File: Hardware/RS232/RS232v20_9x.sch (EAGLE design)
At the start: 13 parts, among them U1 SP3232XTSSOP

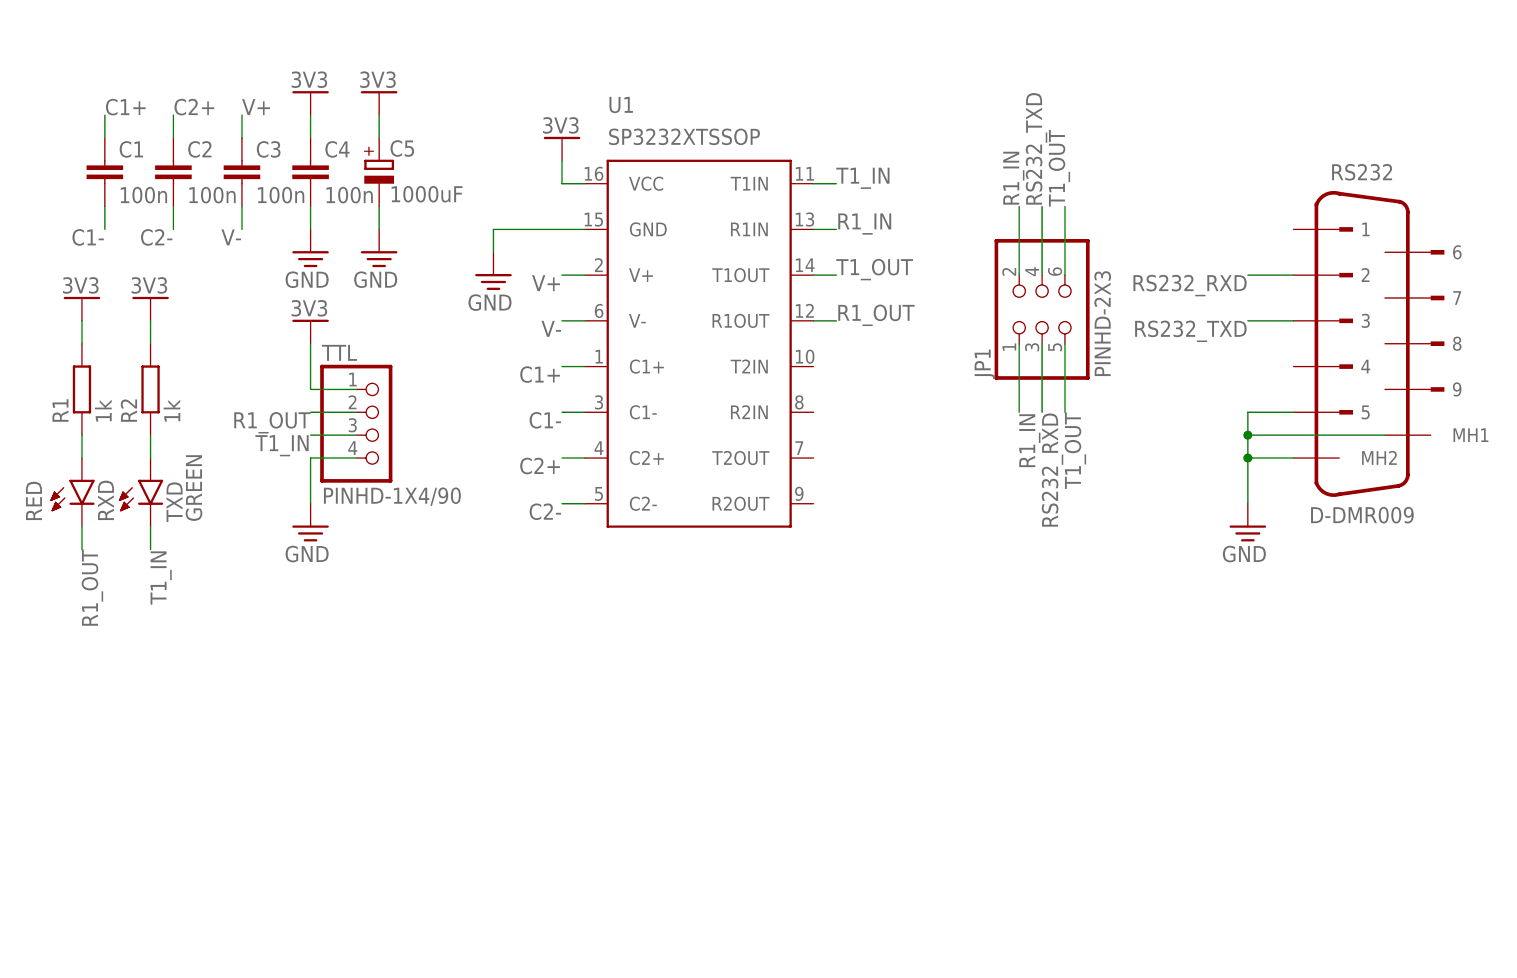
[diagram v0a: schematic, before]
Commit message: RS232 & Powder List
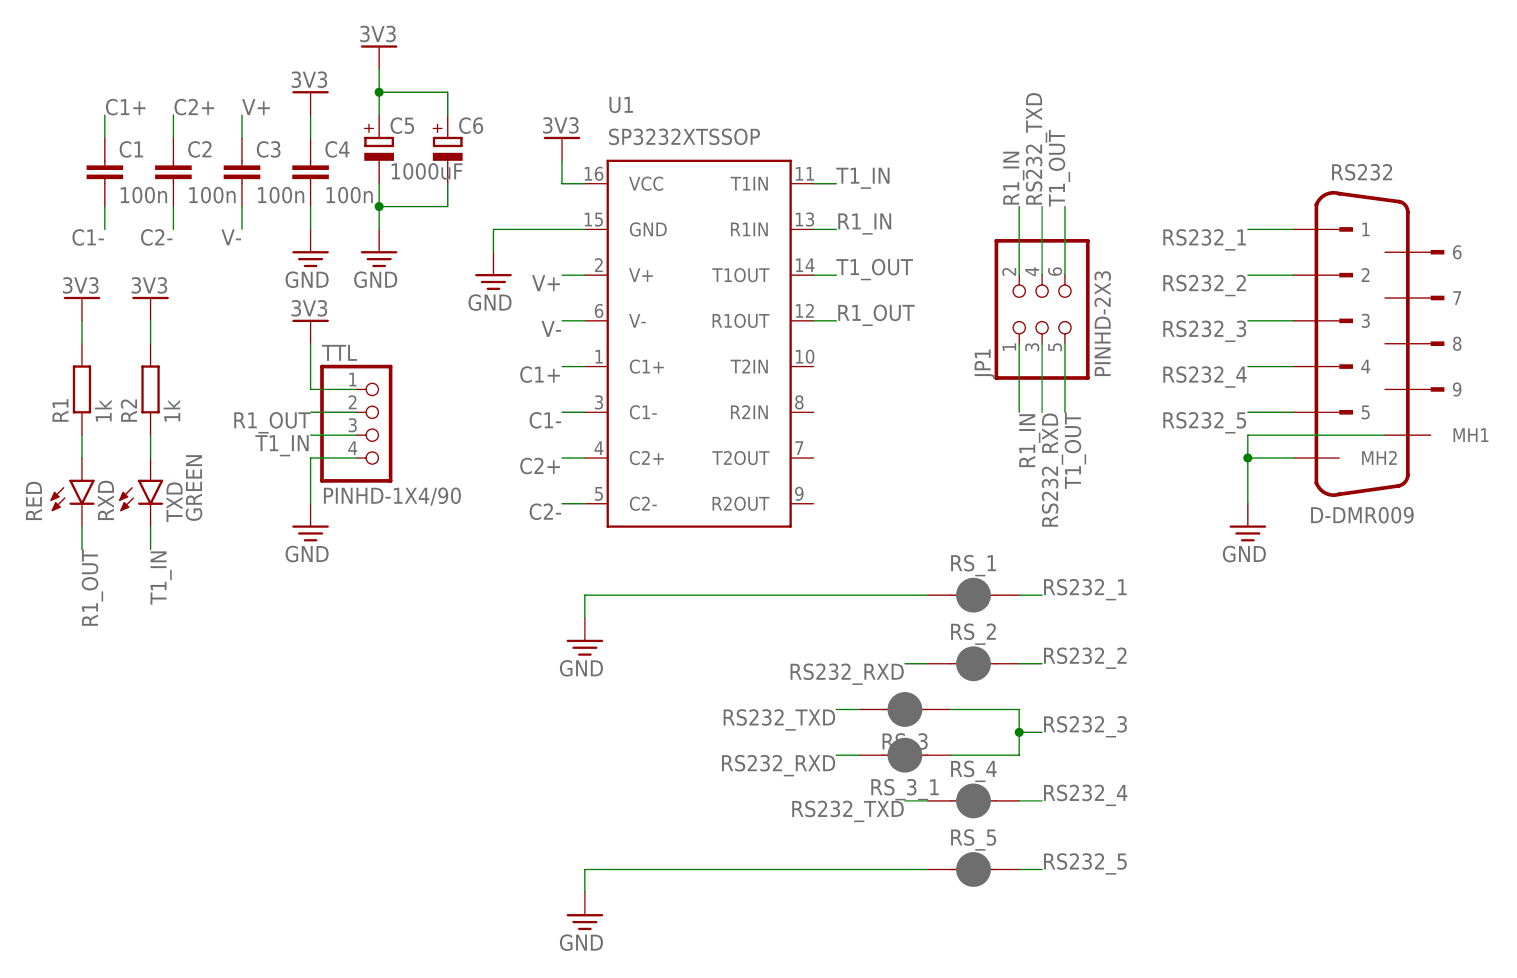
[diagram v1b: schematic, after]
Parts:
- added C6: (no value), Capacitor:C-POL_RADIAL-11MM-DIA
- added RS_1, RS_2, RS_3, RS_3_1, RS_4, RS_5: JUMPER-SMT_2_NC_PASTE_SILK, SparkFun-Jumpers:JUMPER-SMT_2_NC_PASTE_SILK
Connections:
- new net RS232_1: RS232.1, RS_1.2
- new net RS232_2: RS232.2, RS_2.2
- new net RS232_3: RS232.3, RS_3.1, RS_3_1.1
- new net RS232_4: RS232.4, RS_4.2
- new net RS232_5: RS232.5, RS_5.2
- net 3V3: now also C6.+
- net GND: now also C6.-, RS_1.1, RS_5.1; no longer RS232.5
- net RS232_RXD: now also RS_2.1, RS_3_1.2; no longer RS232.2
- net RS232_TXD: now also RS_3.2, RS_4.1; no longer RS232.3
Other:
- moved on the sheet: C5
